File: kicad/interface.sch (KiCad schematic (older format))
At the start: 37 parts, among them P10 C3SB, P11 VSel_Vlv, P14 X_VALVE, P17 PUMP, P18 Pump_Cable, P34 VSel_Vlv2, P38 X_VALVE2, P7 GAGE_PR, P9 C3SB, Q1 BCP5416TA, Q2 BCP5416TA, Q3 BCP5416TA, Q4 BCP5416TA, U1 TXB0104D

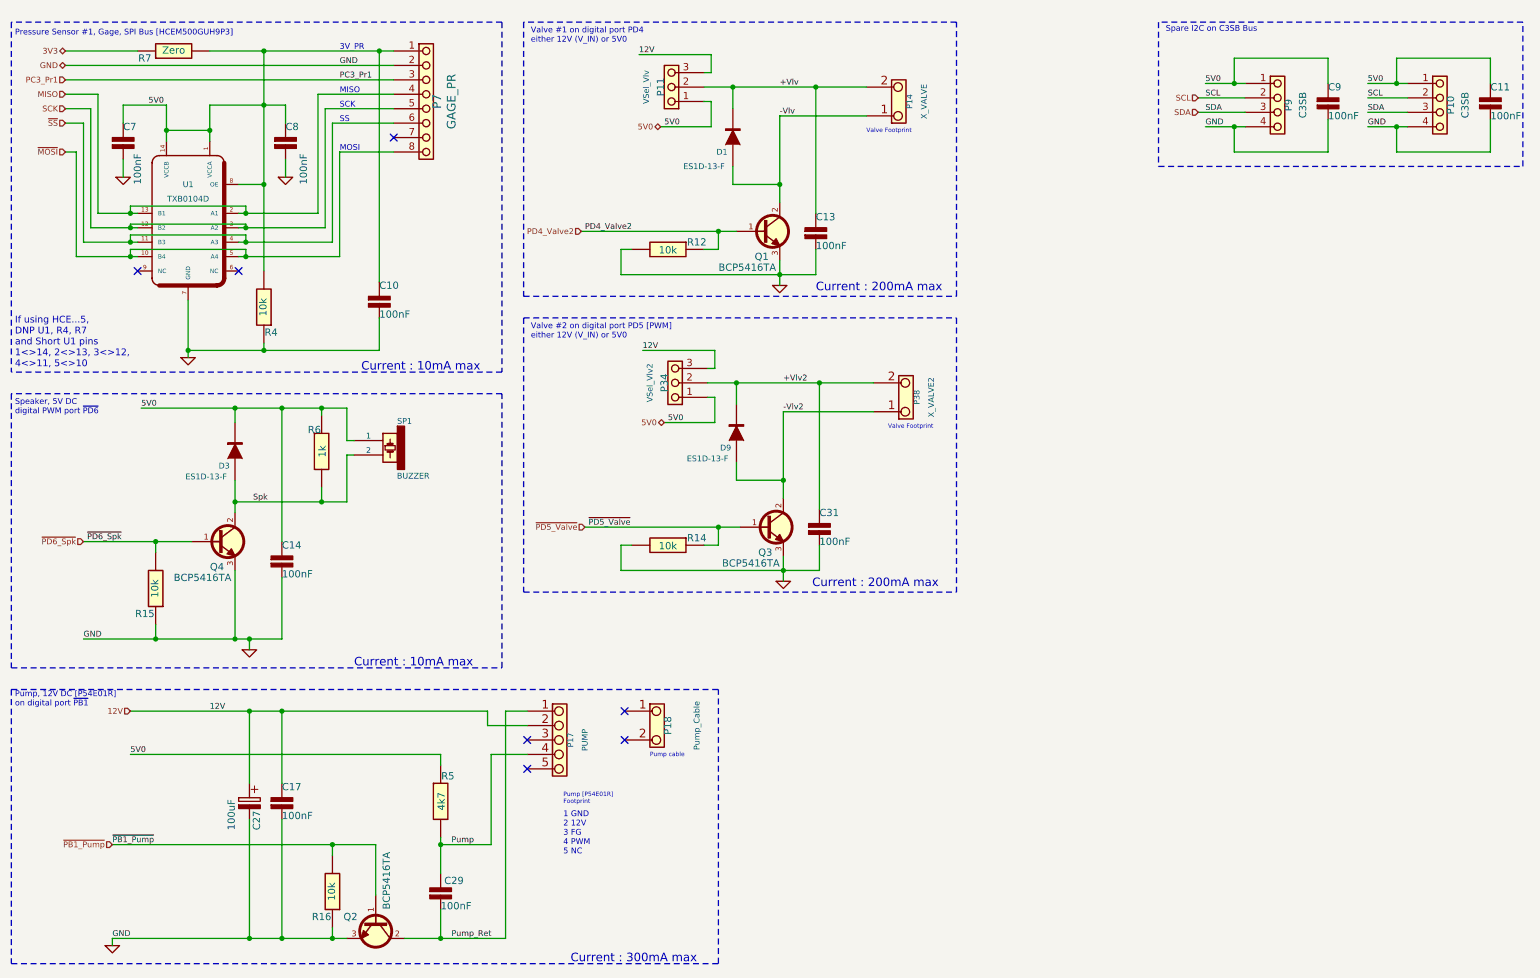
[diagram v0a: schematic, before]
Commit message: made a pretty schematic, fresh symbols
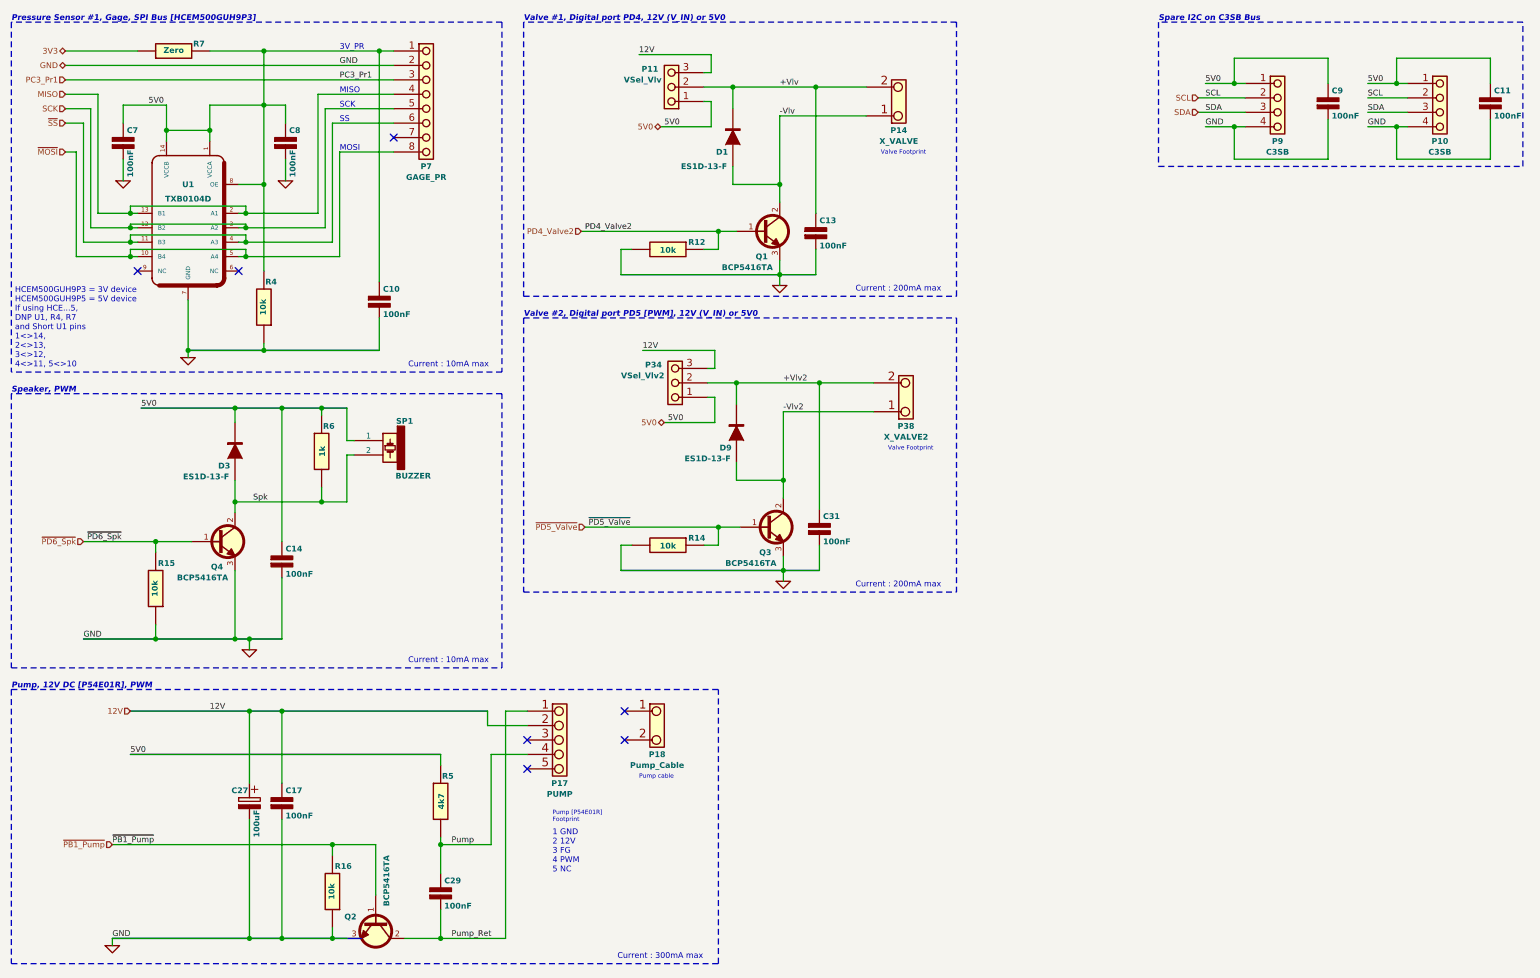
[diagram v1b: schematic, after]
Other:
- note added: "HCEM500GUH9P3 = 3V device\nHCEM500GUH9P5 = 5V device\nIf using HCE...5, \nDNP U1, R4, R7\nand Short U1 pins\n1<>14,\n2<>13,\n3<>12, \n4<>11, 5<>10"
- note added: "Pump, 12V DC [P54E01R], PWM"
- note added: "Speaker, PWM"
- note added: "Valve #1, Digital port PD4, 12V (V_IN) or 5V0"
- note added: "Valve #2, Digital port PD5 [PWM], 12V (V_IN) or 5V0"
- note removed: "If using HCE...5, \nDNP U1, R4, R7\nand Short U1 pins\n1<>14, 2<>13, 3<>12, \n4<>11, 5<>10"
- note removed: "Pump, 12V DC [P54E01R]\non digital port ~PB1"
- note removed: "Speaker, 5V DC\ndigital PWM port ~PD6"
- note removed: "Valve #1 on digital port PD4\neither 12V (V_IN) or 5V0"
- note removed: "Valve #2 on digital port PD5 [PWM]\neither 12V (V_IN) or 5V0"
